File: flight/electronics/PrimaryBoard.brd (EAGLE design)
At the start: 79 x 80.3 mm, 10 parts

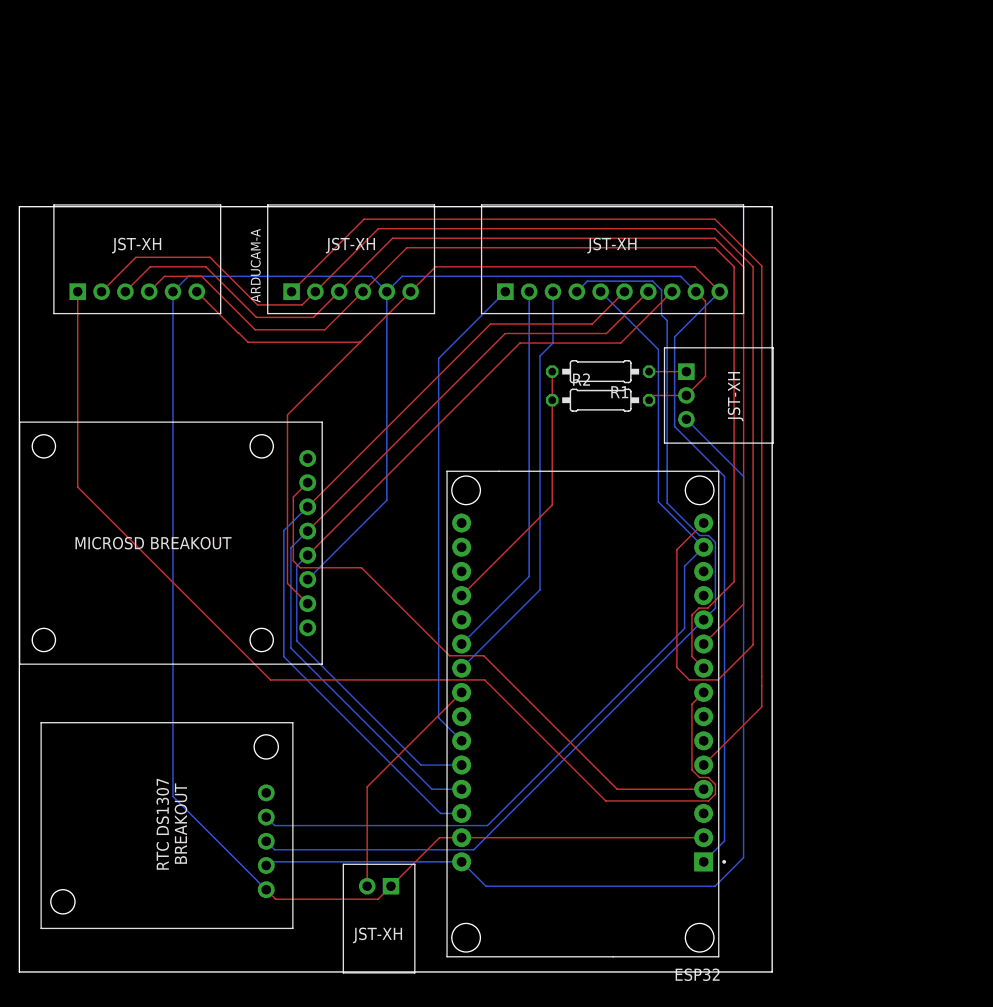
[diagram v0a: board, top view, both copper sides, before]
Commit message: primary board updates
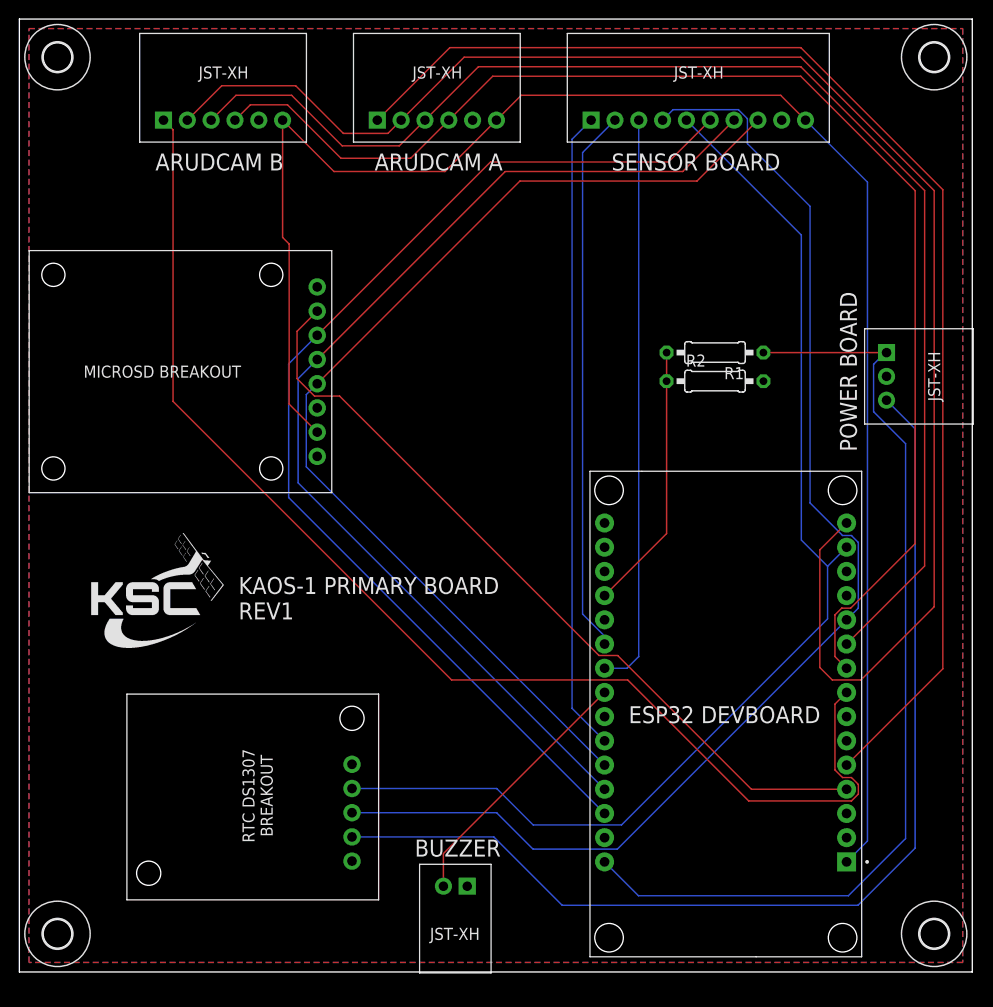
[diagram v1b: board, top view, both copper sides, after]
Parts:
- added U$3, U$4, U$5, U$6: (no value), holes:3,0
- moved POWER_BOARD 21.1 mm to (91.0, 65.0)
- moved ARDUCAM-A 20.1 mm to (37.6, 89.4)
- moved ARDUCAM-B 20.1 mm to (15.1, 89.4)
- moved SENSOR_BOARD 20.1 mm to (60.0, 89.4)
- moved U$1 18.0 mm to (15.0, 63.0)
- moved ESP32 15.0 mm to (74.1, 27.1)
- moved R1 12.2 mm to (73.0, 65.0)
- moved R2 12.2 mm to (73.0, 62.0)
- moved U$2 9.49 mm to (25.0, 19.0)
- moved PIEZO 8.00 mm to (47.0, 9.00)
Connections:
- net +5V: no longer ESP32.30
- net VBAT: now also ESP32.30
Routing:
- net GND: track 223.2 -> 0.00 mm
- net VBAT: track 3.92 -> 101.5 mm
- net HSPI_MOSI: track 84.8 -> 115.7 mm
- net HSPI_MISO: track 83.2 -> 113.4 mm
- net MOSI_CLK: track 81.9 -> 111.2 mm
- net I2C_SCL: track 93.5 -> 121.7 mm
- net I2C_SDA: track 104.0 -> 131.7 mm
- net VSPI_MOSI: track 143.0 -> 166.8 mm
- net VSPI_CLK: track 113.8 -> 137.6 mm
- net VSPI_MISO: track 114.2 -> 138.0 mm
- net ARDUCAM-A_CS: track 109.4 -> 133.2 mm
- net SD_CS: track 61.8 -> 83.5 mm
- net +3V3: track 157.8 -> 177.2 mm
- net ARDUCAM-B_CS: track 114.1 -> 132.3 mm
- net GPIO2: track 39.9 -> 57.3 mm
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- added copper zone on layer 1, net GND
- added copper zone on layer 16, net GND
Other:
- board size 79 x 80.3 mm -> 100 x 100 mm
- board text added: "ARUDCAM A"
- board text added: "ARUDCAM B"
- board text added: "BUZZER"
- board text added: "ESP32 DEVBOARD"
- board text added: "KAOS-1 PRIMARY BOARD REV1"
- board text added: "POWER BOARD"
- board text added: "SENSOR BOARD"
